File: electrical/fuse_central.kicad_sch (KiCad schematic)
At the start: 1 part, among them U5 ROLL TRIM

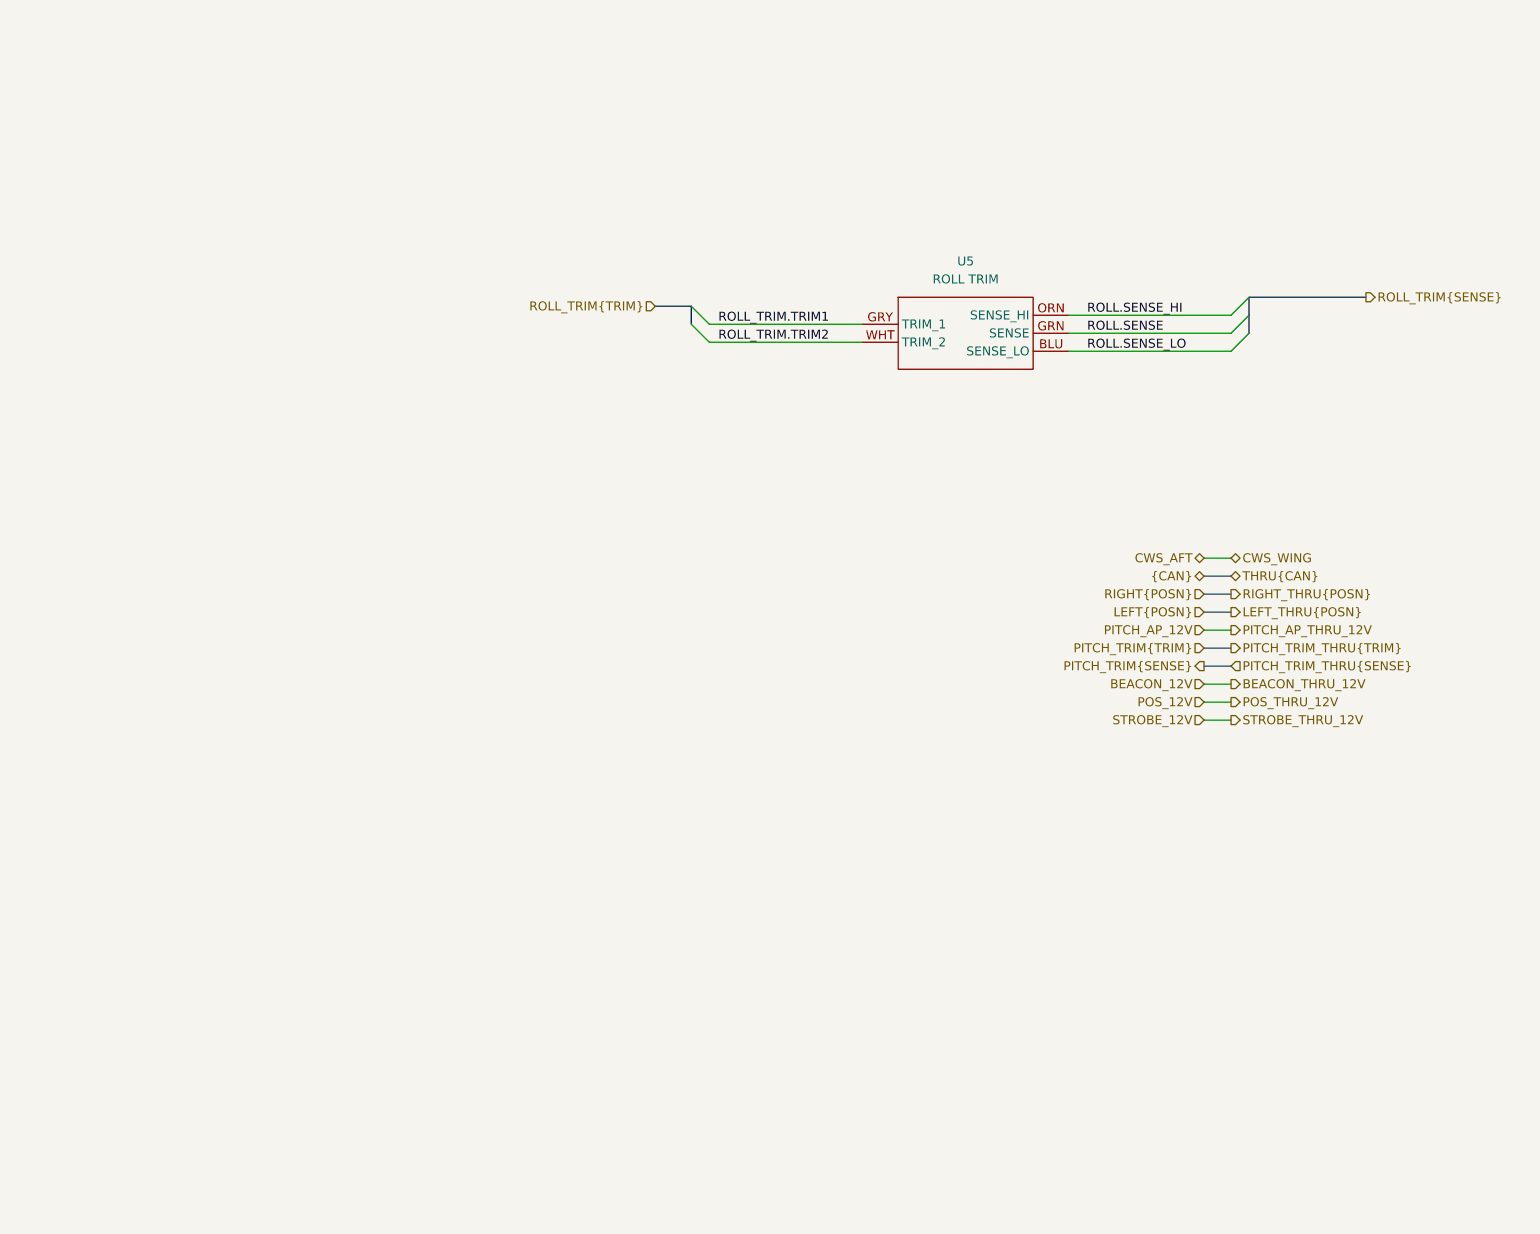
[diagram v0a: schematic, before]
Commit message: 🎮 Working on electrical schematic
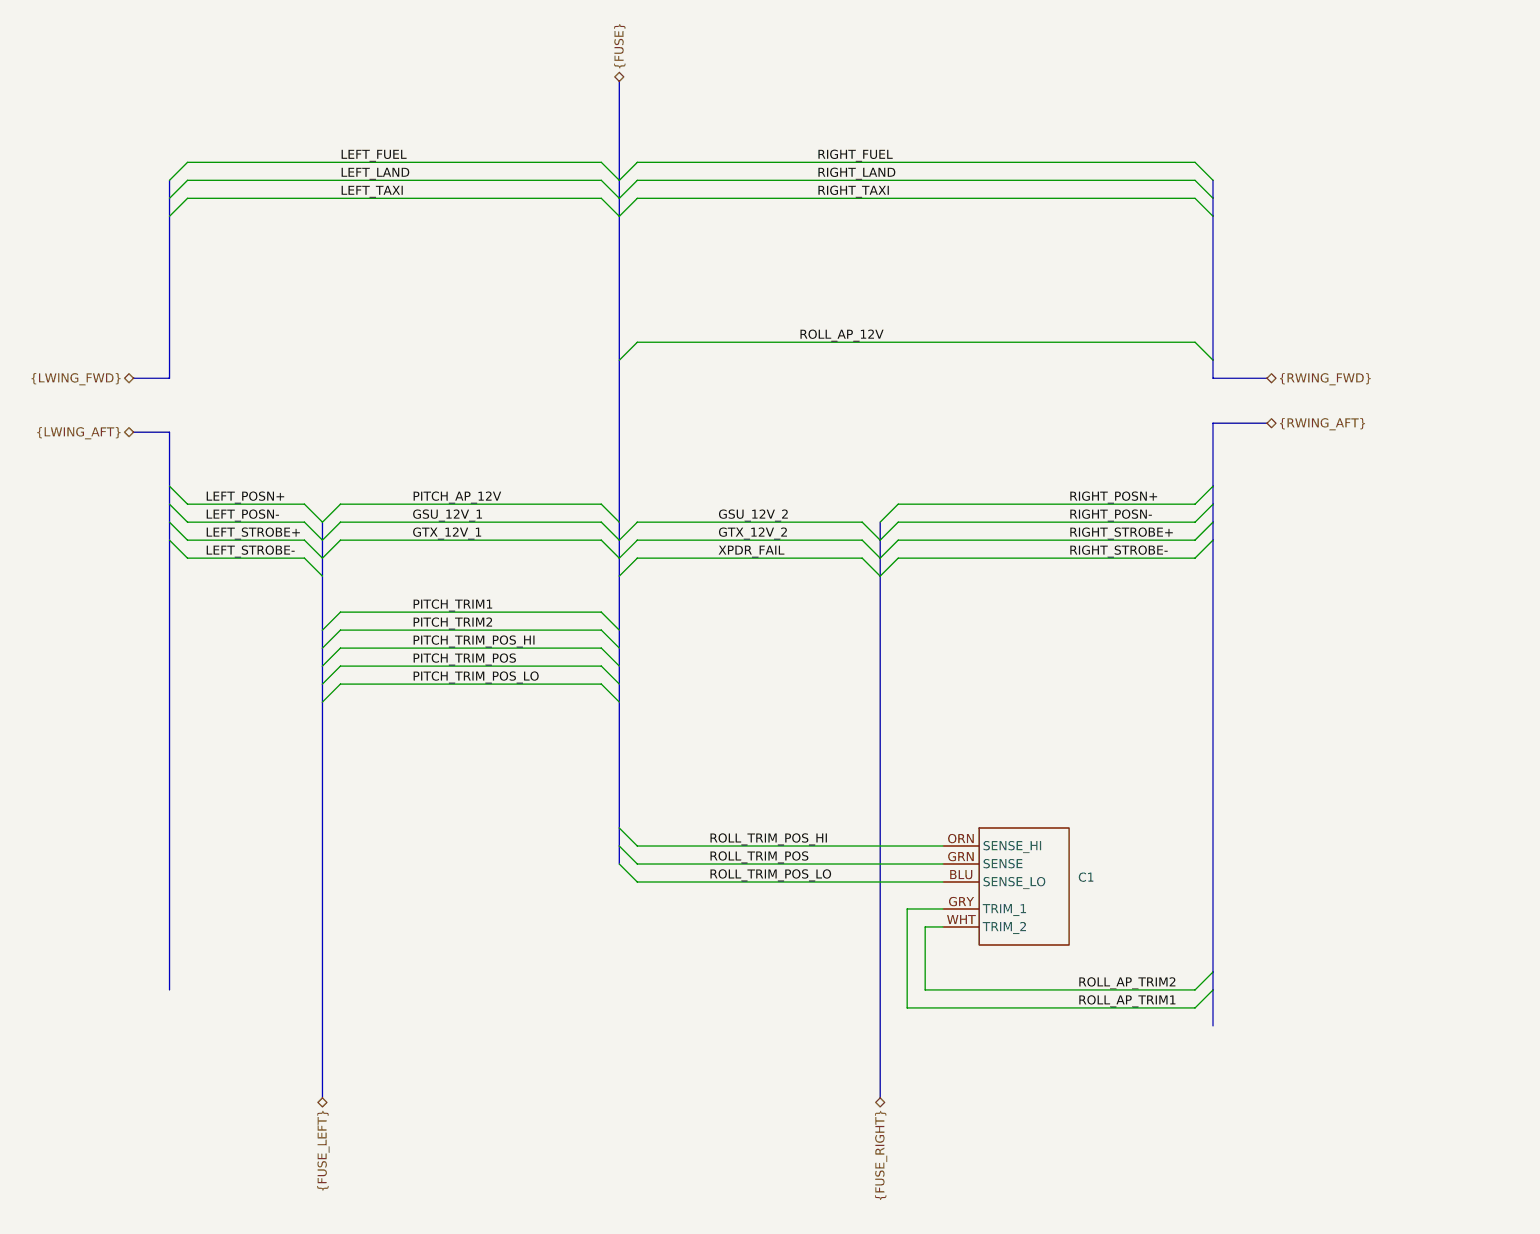
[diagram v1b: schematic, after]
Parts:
- renumbered U5 to C1
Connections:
- net ROLL.SENSE renamed ROLL_TRIM_POS
- net ROLL.SENSE_HI renamed ROLL_TRIM_POS_HI
- net ROLL.SENSE_LO renamed ROLL_TRIM_POS_LO
- net ROLL_TRIM.TRIM1 renamed ROLL_AP_TRIM1
- net ROLL_TRIM.TRIM2 renamed ROLL_AP_TRIM2
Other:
- moved on the sheet: C1
